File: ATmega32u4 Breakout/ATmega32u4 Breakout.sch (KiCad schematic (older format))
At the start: 6 parts, among them J1 Conn_01x22_Male, J2 Conn_01x22_Male, U1 ATmega32U4-AU, Y1 16MHz

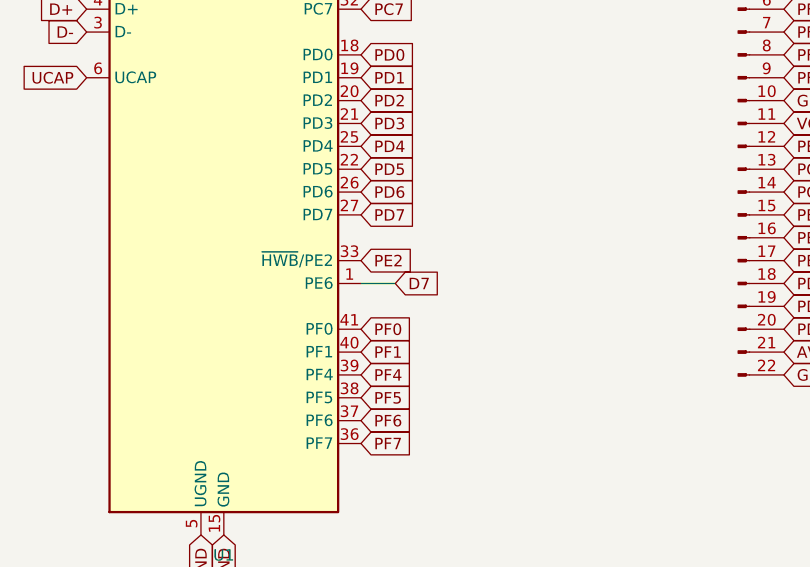
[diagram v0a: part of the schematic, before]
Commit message: Lots of work over the weekend.
Nearly done, gerber files made too.  I think it's ready to be turned into PCB.
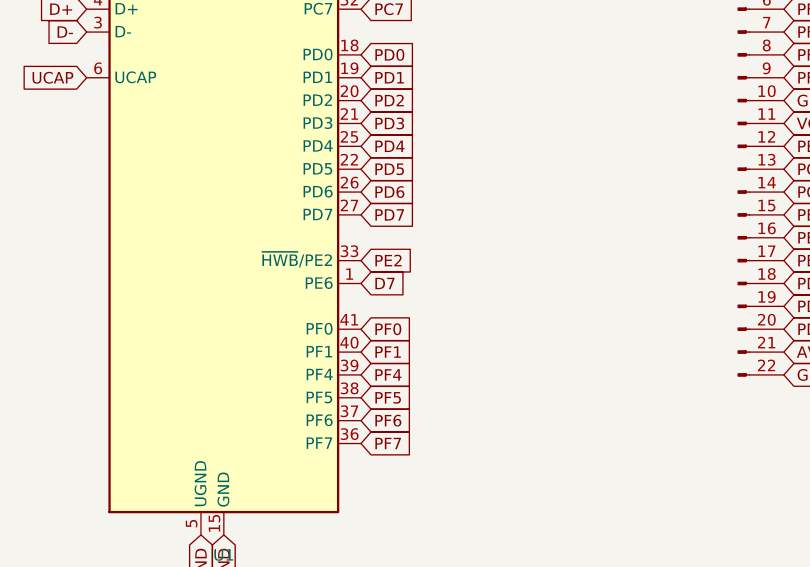
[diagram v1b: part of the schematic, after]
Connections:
- wire segments 11 -> 10
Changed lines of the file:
@@
 	1    0    0    -1
 $EndComp
-Wire Wire Line
-	6350 4200 6500 4200
-Text GLabel 6500 4200 2    50   Input ~ 0
+Text GLabel 6350 4200 2    50   Input ~ 0
 D7
 Text GLabel 3200 2500 2    50   Input ~ 0
